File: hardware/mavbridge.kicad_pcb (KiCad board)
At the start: 2 copper layers, 35 x 25 mm, 25 parts, among them P1 PX4, P2 DEBUG, P3 PWR, U1 ESP-12E, U2 AP7361

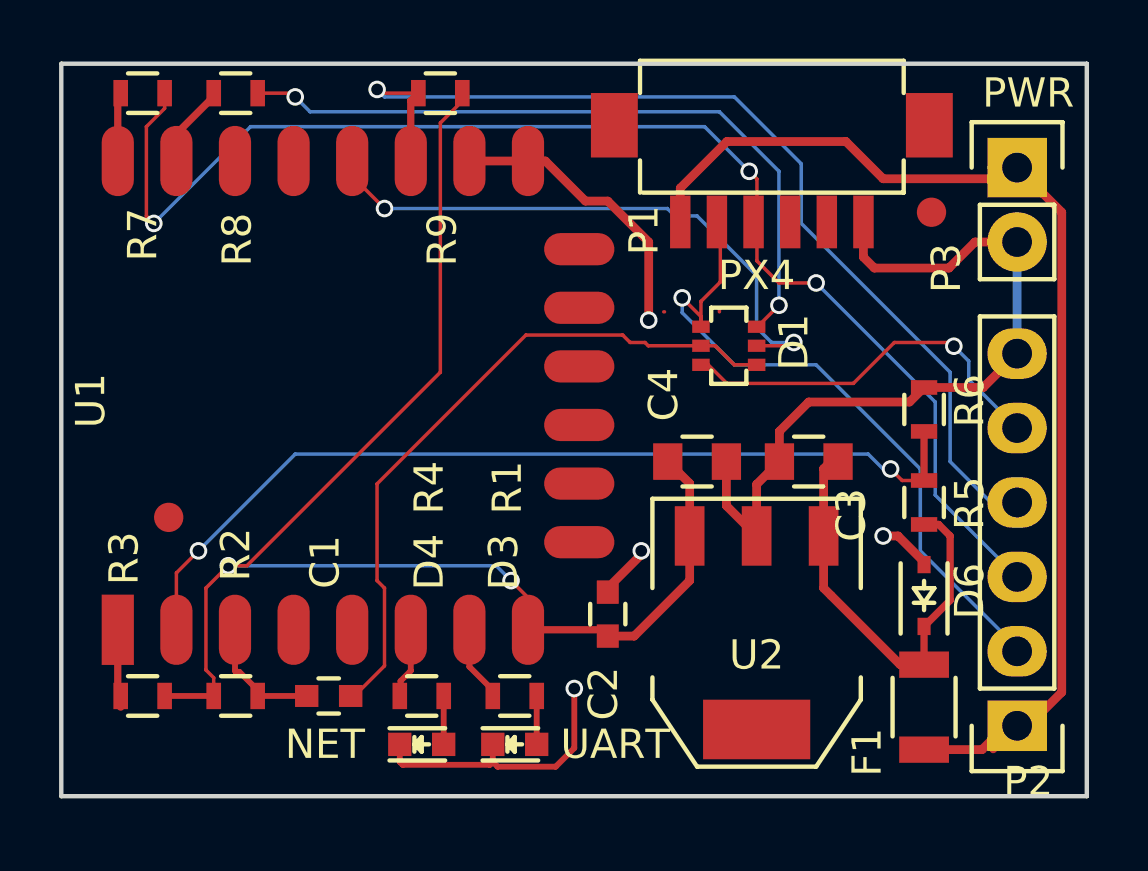
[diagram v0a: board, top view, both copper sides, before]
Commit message: Ordered rev2 hardware.
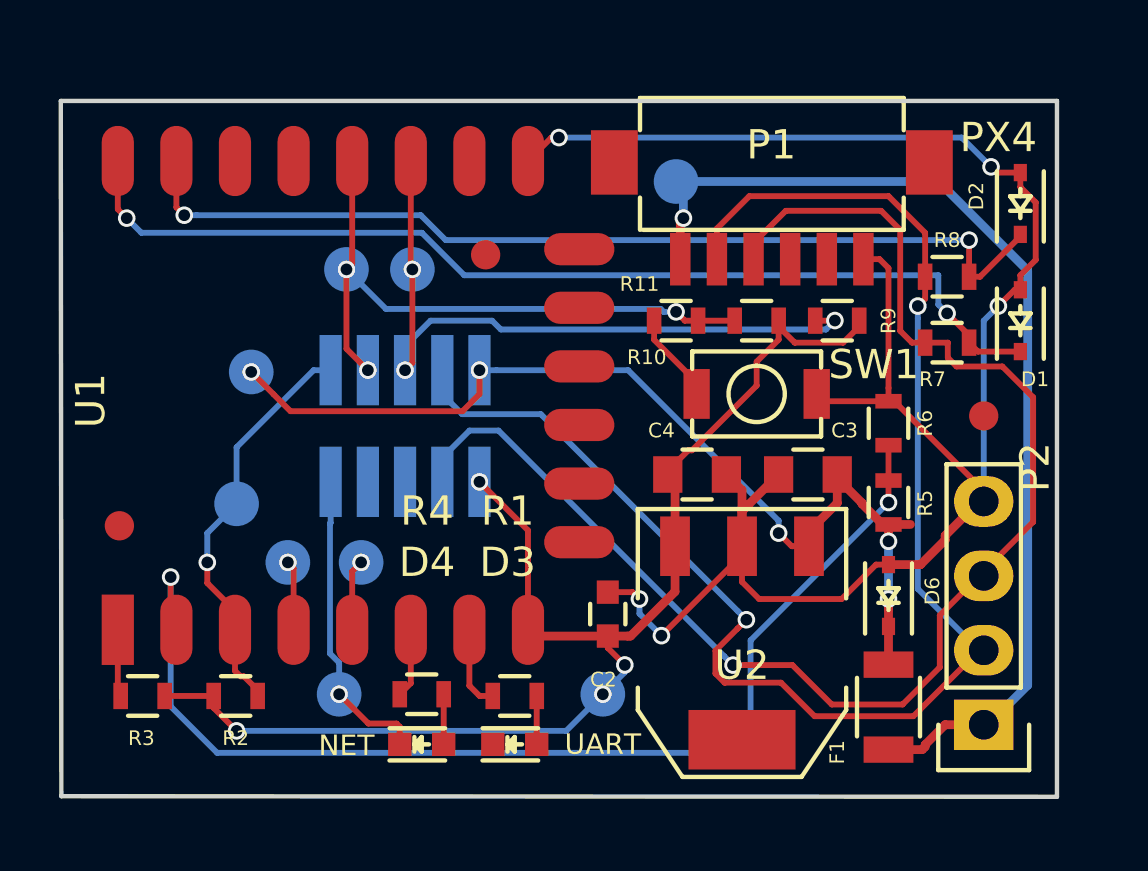
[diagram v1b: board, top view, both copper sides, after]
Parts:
- removed C1: 0.1uF, Capacitors_SMD:C_0603
- removed the REF** at (194.2, 116.7)
- removed the REF** at (219.7, 106.3)
- added D2: ZENERsmall, Diodes_SMD:SOD-323, F.Cu at (223.2, 106.0)
- added R10: 10K, Resistors_SMD:R_0603, F.Cu at (214.2, 110.0)
- added R11: 120R, Resistors_SMD:R_0603, F.Cu at (211.5, 110.0)
- added REF**: FIDUCIAL, manufacturing:FIDUCIAL, F.Cu at (192.5, 117.0)
- added REF**: FIDUCIAL, manufacturing:FIDUCIAL, F.Cu at (205.0, 107.8)
- added REF**: FIDUCIAL, manufacturing:FIDUCIAL, F.Cu at (222.0, 113.2)
- added SW1: SW_PUSH, tact_switch:TACT_SW_TACTD44H20B160, F.Cu at (214.2, 112.5)
- added W1: TEST_1P, Measurement_Points:Measurement_Point_Round-SMD-Pad_Small, B.Cu at (209.0, 122.8)
- added W2: TEST_1P, Measurement_Points:Measurement_Point_Round-SMD-Pad_Small, B.Cu at (197.0, 111.8)
- added W3: TEST_1P, Measurement_Points:Measurement_Point_Round-SMD-Pad_Small, B.Cu at (200.0, 122.8)
- added W4: TEST_1P, Measurement_Points:Measurement_Point_Round-SMD-Pad_Small, B.Cu at (200.2, 108.2)
- added W5: TEST_1P, Measurement_Points:Measurement_Point_Round-SMD-Pad_Small, B.Cu at (196.5, 116.2)
- added W6: TEST_1P, Measurement_Points:Measurement_Point_Round-SMD-Pad_Small, B.Cu at (198.2, 118.2)
- added W7: TEST_1P, Measurement_Points:Measurement_Point_Round-SMD-Pad_Small, B.Cu at (200.8, 118.2)
- added W8: TEST_1P, Measurement_Points:Measurement_Point_Round-SMD-Pad_Small, B.Cu at (202.5, 108.2)
- added W9: TEST_1P, Measurement_Points:Measurement_Point_Round-SMD-Pad_Small, B.Cu at (211.5, 105.2)
- D1: value BAT54TW -> ZENERsmall; footprint sot363:SOT-363 -> Diodes_SMD:SOD-323
- P2: value DEBUG -> UART; footprint Pin_Headers:Pin_Header_Straight_1x06 -> Pin_Headers:Pin_Header_Straight_1x04
- P3: value PWR -> CONN_02X05; footprint Pin_Headers:Pin_Header_Straight_1x02 -> pin_headers_1.27mm:Pin_Header_1.27mm_2x5; moved to B.Cu
- moved R7 28.7 mm to (220.8, 110.8), turned to 0 degrees
- moved R8 25.1 mm to (220.8, 108.5), turned to 0 degrees
- moved P3 21.3 mm to (204.8, 115.5), turned to 90 degrees
- moved R9 15.6 mm to (217.0, 110.0)
- moved D1 9.13 mm to (223.2, 110.0), turned to 90 degrees
- moved R6 1.30 mm to (218.8, 113.5)
- moved P1 1.27 mm to (214.8, 107.0)
- moved D6 1.21 mm to (218.8, 119.4)
- moved F1 1.21 mm to (218.8, 123.2)
- moved R5 1.21 mm to (218.8, 116.2)
- moved P2 1.14 mm to (222.0, 123.8)
- moved U2 0.61 mm to (213.8, 121.0)
- moved C3 0.44 mm to (216.0, 115.2)
- moved C4 0.44 mm to (212.2, 115.2)
- moved R4 0.06 mm to (202.8, 122.8)
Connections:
- D1 pad 1: Net-(C1-Pad2) -> Net-(D1-Pad1)
- D1 pad 2: /GPIO0 -> GND
- P2 pad 4: /DBG_TX -> GND
- P3 pad 1: VPP -> +3V3
- P3 pad 2: GND -> +5V
- R2 pad 1: Net-(C1-Pad1) -> /CH_PD
- R7 pad 2: Net-(R7-Pad2) -> Net-(D1-Pad1)
- R8 pad 1: Net-(D1-Pad3) -> RXD
- U1 pad 22: Net-(R7-Pad2) -> Net-(D1-Pad1)
- U1 pad 3: Net-(C1-Pad1) -> /CH_PD
- U1 pad 4: (no net) -> /GPIO16
- U1 pad 5: (no net) -> /GPIO14
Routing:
- net Net-(D1-Pad1): track 0.00 -> 35.2 mm, vias 0 -> 2
- net Net-(D2-Pad1): track 2.84 -> 32.7 mm, vias 0 -> 2
- net RXD: track 23.2 -> 51.9 mm, vias 1 -> 2
- net GND: track 50.6 -> 77.1 mm, vias 4 -> 6
- net Net-(D1-Pad3): track 24.5 -> 0.00 mm, vias 2 -> 0
- net Net-(C1-Pad2): track 23.4 -> 0.00 mm
- net +5V: track 15.4 -> 34.3 mm, vias 0 -> 5
- net DTR: track 14.1 -> 0.00 mm, vias 1 -> 0
- net /CH_PD: track 0.00 -> 14.0 mm, vias 0 -> 1
- net /DBG_TX: track 34.5 -> 24.0 mm, vias 1 -> 3
- net Net-(R5-Pad1): track 31.2 -> 40.5 mm
- net VPP: track 41.0 -> 35.9 mm, vias 0 -> 1
- net +3V3: track 49.3 -> 44.8 mm, vias 2 -> 4
- net Net-(C1-Pad1): track 4.32 -> 0.00 mm
- net TXD: track 45.5 -> 48.8 mm, vias 3 -> 1
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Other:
- board size 35 x 25 mm -> 34 x 23.8 mm
- board text added: "MAVLink WiFi bridge rev. 2"
- board text removed: "DBG_TX"
- board text removed: "DTR"
- board text removed: "MAVLink WiFi bridge rev. 1"
